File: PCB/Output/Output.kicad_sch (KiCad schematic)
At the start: 64 parts, among them J1 POWER, J10 O7, J11 O8, J12 O9, J13 O10, J2 Shelly, J2 USB-C, J4 O1, J5 O2, J6 O3, J7 O4, J8 O5, J9 O6, U1 MD8942, U2 ESP32-S3-MINI-1, U3 ISL89410, U4 ISL89410, U5 ISL89410, U6 ISL89410, U7 ISL89410

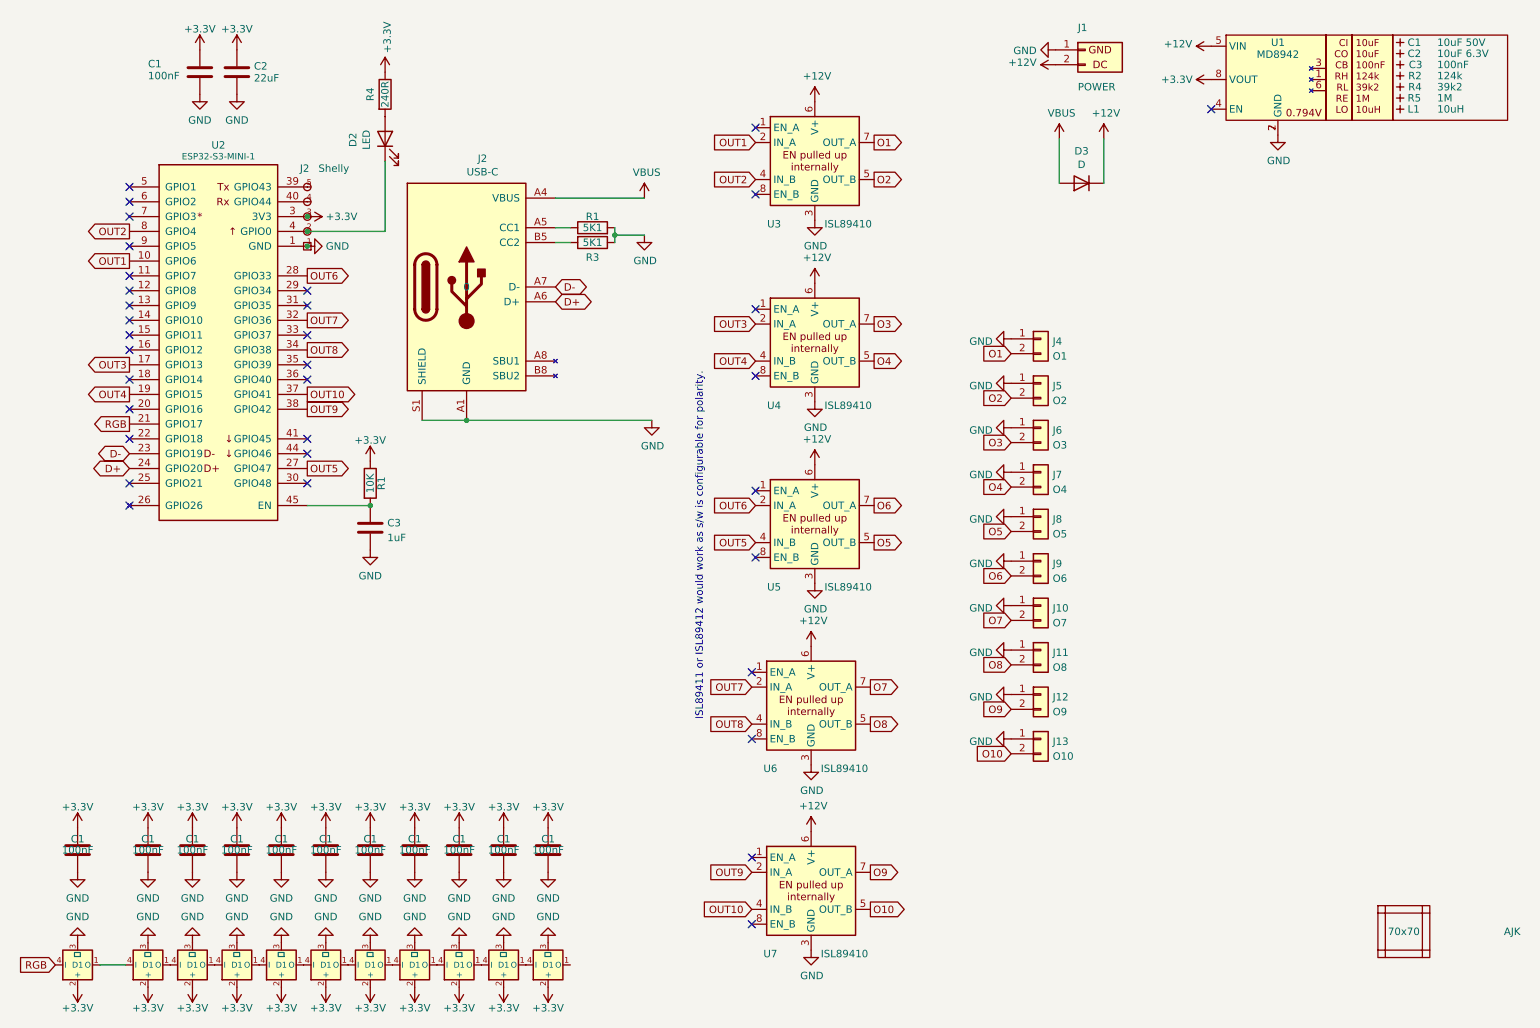
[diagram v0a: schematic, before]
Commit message: Library update
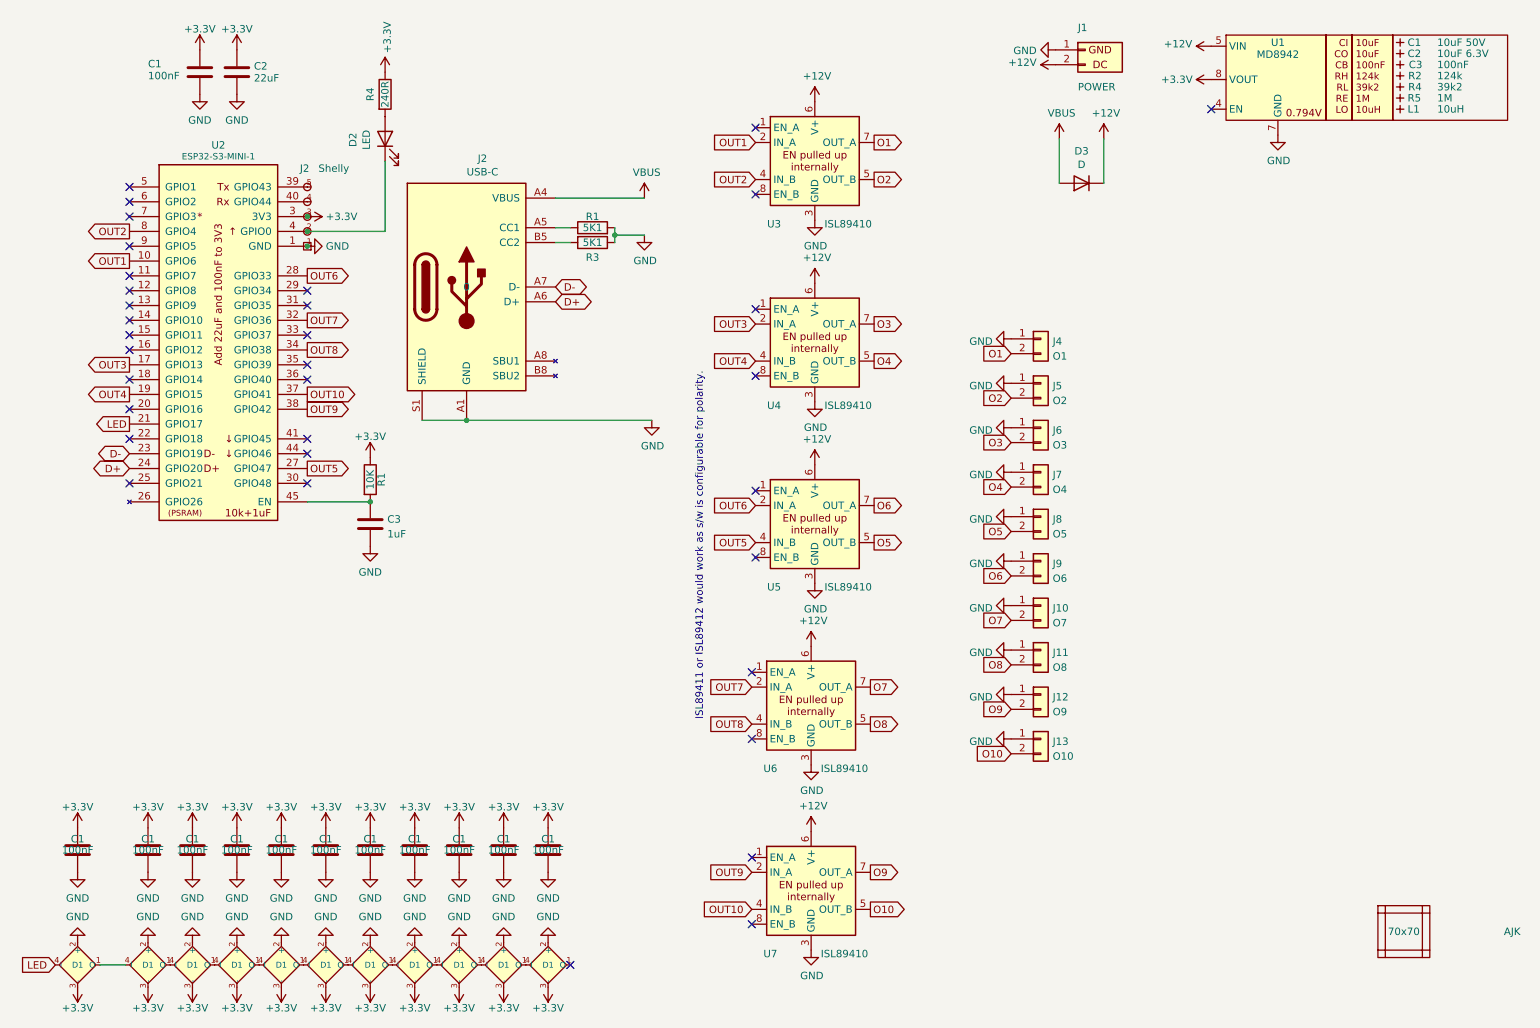
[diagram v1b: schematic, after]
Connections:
- net +3.3V: now also D1.3 (-), D1.3 (-), D1.3 (-), D1.3 (-), D1.3 (-), D1.3 (-), D1.3 (-), D1.3 (-), D1.3 (-), D1.3 (-), D1.3 (-); no longer D1.2 (+), D1.2 (+), D1.2 (+), D1.2 (+), D1.2 (+), D1.2 (+), D1.2 (+), D1.2 (+), D1.2 (+), D1.2 (+), D1.2 (+)
- net GND: now also D1.2 (+), D1.2 (+), D1.2 (+), D1.2 (+), D1.2 (+), D1.2 (+), D1.2 (+), D1.2 (+), D1.2 (+), D1.2 (+), D1.2 (+); no longer D1.3 (⏚), D1.3 (⏚), D1.3 (⏚), D1.3 (⏚), D1.3 (⏚), D1.3 (⏚), D1.3 (⏚), D1.3 (⏚), D1.3 (⏚), D1.3 (⏚), D1.3 (⏚)
- net RGB renamed LED
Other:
- moved on the sheet: C3, R1
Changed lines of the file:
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@@
   (junction (at 68.58 52.705) (diameter 0) (color 0 0 0 0)
   )
-  (junction (at 79.375 102.235) (diameter 0) (color 0 0 0 0)
+  (junction (at 79.375 101.6) (diameter 0) (color 0 0 0 0)
   )
   (junction (at 121.285 55.88) (diameter 0) (color 0 0 0 0)
@@
   (no_connect (at 38.1 73.025))
   (no_connect (at 38.1 52.705))
-  (no_connect (at 38.1 102.235))
+  (no_connect (at 113.665 180.975))
   (no_connect (at 38.1 65.405))
   (no_connect (at 38.1 90.805))
@@
     (stroke (width 0) (type default))
   )
-  (wire (pts (xy 68.58 102.235) (xy 79.375 102.235))
+  (wire (pts (xy 68.58 101.6) (xy 79.375 101.6))
     (stroke (width 0) (type default))
   )
@@
     )
   )
-  (global_label "RGB" (shape input) (at 25.4 180.975 180) (fields_autoplaced)
+  (global_label "LED" (shape input) (at 25.4 180.975 180) (fields_autoplaced)
     (effects (font (size 1.27 1.27)) (justify right))
-    (property "Intersheetrefs" "${INTERSHEET_REFS}" (at 19.259 180.975 0)
+    (property "Intersheetrefs" "${INTERSHEET_REFS}" (at 19.6219 180.975 0)
       (effects (font (size 1.27 1.27)) (justify right) hide)
     )
@@
     )
   )
-  (global_label "RGB" (shape output) (at 38.1 88.265 180) (fields_autoplaced)
+  (global_label "LED" (shape output) (at 38.1 88.265 180) (fields_autoplaced)
     (effects (font (size 1.27 1.27)) (justify right))
-    (property "Intersheetrefs" "${INTERSHEET_REFS}" (at 31.959 88.265 0)
+    (property "Intersheetrefs" "${INTERSHEET_REFS}" (at 32.3219 88.265 0)
       (effects (font (size 1.27 1.27)) (justify right) hide)
     )
@@
       (effects (font (size 1.27 1.27)) hide)
     )
+    (property "Part No" "" (at 255.905 32.385 0)
+      (effects (font (size 1.27 1.27)) hide)
+    )
+    (property "Note" "" (at 255.905 32.385 0)
+      (effects (font (size 1.27 1.27)) hide)
+    )
     (pin "~")
     (instances
@@
       (effects (font (size 1.27 1.27)) hide)
     )
+    (property "Part No" "" (at 255.905 30.48 0)
+      (effects (font (size 1.27 1.27)) hide)
+    )
+    (property "Note" "" (at 255.905 30.48 0)
+      (effects (font (size 1.27 1.27)) hide)
+    )
     (pin "~")
     (instances
@@
     )
   )
-  (symbol (lib_id "Device:C") (at 79.375 106.045 0) (unit 1)
+  (symbol (lib_id "Device:C") (at 79.375 105.41 0) (unit 1)
     (in_bom yes) (on_board yes) (dnp no) (fields_autoplaced)
-    (property "Reference" "C3" (at 82.296 105.2103 0)
+    (property "Reference" "C3" (at 82.296 104.5753 0)
       (effects (font (size 1.27 1.27)) (justify left))
     )
-    (property "Value" "1uF" (at 82.296 107.7472 0)
+    (property "Value" "1uF" (at 82.296 107.1122 0)
       (effects (font (size 1.27 1.27)) (justify left))
     )
-    (property "Footprint" "RevK:C_0402" (at 80.3402 109.855 0)
+    (property "Footprint" "RevK:C_0402" (at 80.3402 109.22 0)
       (effects (font (size 1.27 1.27)) hide)
     )
-    (property "Datasheet" "~" (at 79.375 106.045 0)
+    (property "Datasheet" "~" (at 79.375 105.41 0)
       (effects (font (size 1.27 1.27)) hide)
     )
@@
       (effects (font (size 1.27 1.27)) hide)
     )
+    (property "Part No" "" (at 255.905 24.765 0)
+      (effects (font (size 1.27 1.27)) hide)
+    )
+    (property "Note" "" (at 255.905 24.765 0)
+      (effects (font (size 1.27 1.27)) hide)
+    )
     (pin "~")
     (instances
@@
       (effects (font (size 1.27 1.27)) hide)
     )
+    (property "Part No" "" (at 255.905 22.86 0)
+      (effects (font (size 1.27 1.27)) hide)
+    )
+    (property "Note" "" (at 255.905 22.86 0)
+      (effects (font (size 1.27 1.27)) hide)
+    )
     (pin "~")
     (instances
@@
       (effects (font (size 1.27 1.27)) hide)
     )
+    (property "Part No" "" (at 255.905 28.575 0)
+      (effects (font (size 1.27 1.27)) hide)
+    )
+    (property "Note" "" (at 255.905 28.575 0)
+      (effects (font (size 1.27 1.27)) hide)
+    )
     (pin "~")
     (instances
@@
     )
   )
-  (symbol (lib_id "power:+3.3V") (at 79.375 94.615 0) (unit 1)
+  (symbol (lib_id "power:+3.3V") (at 79.375 93.98 0) (unit 1)
     (in_bom yes) (on_board yes) (dnp no) (fields_autoplaced)
-    (property "Reference" "#PWR0106" (at 79.375 98.425 0)
+    (property "Reference" "#PWR0106" (at 79.375 97.79 0)
       (effects (font (size 1.27 1.27)) hide)
     )
-    (property "Value" "+3.3V" (at 79.375 91.0392 0)
+    (property "Value" "+3.3V" (at 79.375 90.4042 0)
       (effects (font (size 1.27 1.27)))
     )
-    (property "Footprint" "" (at 79.375 94.615 0)
+    (property "Footprint" "" (at 79.375 93.98 0)
       (effects (font (size 1.27 1.27)) hide)
     )
-    (property "Datasheet" "" (at 79.375 94.615 0)
+    (property "Datasheet" "" (at 79.375 93.98 0)
       (effects (font (size 1.27 1.27)) hide)
     )
@@
     )
   )
-  (symbol (lib_id "Device:R") (at 79.375 98.425 0) (unit 1)
+  (symbol (lib_id "Device:R") (at 79.375 97.79 0) (unit 1)
     (in_bom yes) (on_board yes) (dnp no)
-    (property "Reference" "R1" (at 81.28 98.425 90)
+    (property "Reference" "R1" (at 81.28 97.79 90)
       (effects (font (size 1.27 1.27)))
     )
-    (property "Value" "10K" (at 79.375 98.425 90)
+    (property "Value" "10K" (at 79.375 97.79 90)
       (effects (font (size 1.27 1.27)))
     )
-    (property "Footprint" "RevK:R_0402" (at 77.597 98.425 90)
+    (property "Footprint" "RevK:R_0402" (at 77.597 97.79 90)
       (effects (font (size 1.27 1.27)) hide)
     )
-    (property "Datasheet" "~" (at 79.375 98.425 0)
+    (property "Datasheet" "~" (at 79.375 97.79 0)
       (effects (font (size 1.27 1.27)) hide)
     )
@@
     )
   )
-  (symbol (lib_id "power:GND") (at 79.375 109.855 0) (unit 1)
+  (symbol (lib_id "power:GND") (at 79.375 109.22 0) (unit 1)
     (in_bom yes) (on_board yes) (dnp no) (fields_autoplaced)
-    (property "Reference" "#PWR0105" (at 79.375 116.205 0)
+    (property "Reference" "#PWR0105" (at 79.375 115.57 0)
       (effects (font (size 1.27 1.27)) hide)
     )
-    (property "Value" "GND" (at 79.375 114.2984 0)
+    (property "Value" "GND" (at 79.375 113.6634 0)
       (effects (font (size 1.27 1.27)))
     )
-    (property "Footprint" "" (at 79.375 109.855 0)
+    (property "Footprint" "" (at 79.375 109.22 0)
       (effects (font (size 1.27 1.27)) hide)
     )
-    (property "Datasheet" "" (at 79.375 109.855 0)
+    (property "Datasheet" "" (at 79.375 109.22 0)
       (effects (font (size 1.27 1.27)) hide)
     )
@@
       (effects (font (size 1.27 1.27)) hide)
     )
+    (property "Part No" "" (at 255.905 26.67 0)
+      (effects (font (size 1.27 1.27)) hide)
+    )
+    (property "Note" "" (at 255.905 26.67 0)
+      (effects (font (size 1.27 1.27)) hide)
+    )
     (pin "~")
     (instances
@@
       (effects (font (size 1.27 1.27)) hide)
     )
+    (property "Sim.Device" "D" (at 201.295 46.99 0)
+      (effects (font (size 1.27 1.27)) hide)
+    )
+    (property "Sim.Pins" "1=K 2=A" (at 201.295 46.99 0)
+      (effects (font (size 1.27 1.27)) hide)
+    )
     (pin "1")
     (pin "2")
@@
       (effects (font (size 1.27 1.27)) hide)
     )
+    (property "Part No" "" (at 255.905 34.29 0)
+      (effects (font (size 1.27 1.27)) hide)
+    )
+    (property "Note" "" (at 255.905 34.29 0)
+      (effects (font (size 1.27 1.27)) hide)
+    )
     (pin "~")
     (instances
@@
     )
   )
-  (symbol (lib_name "GND_1") (lib_id "power:GND") (at 68.58 57.785 90) (unit 1)
+  (symbol (lib_id "power:GND") (at 68.58 57.785 90) (unit 1)
     (in_bom yes) (on_board yes) (dnp no) (fields_autoplaced)
     (property "Reference" "#PWR01" (at 74.93 57.785 0)
